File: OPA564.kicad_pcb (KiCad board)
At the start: 2 copper layers, 57.5 x 55 mm, 15 parts, among them IC1 OPA564AIDWD, J1 Conn_Coaxial, J2 Conn_Coaxial

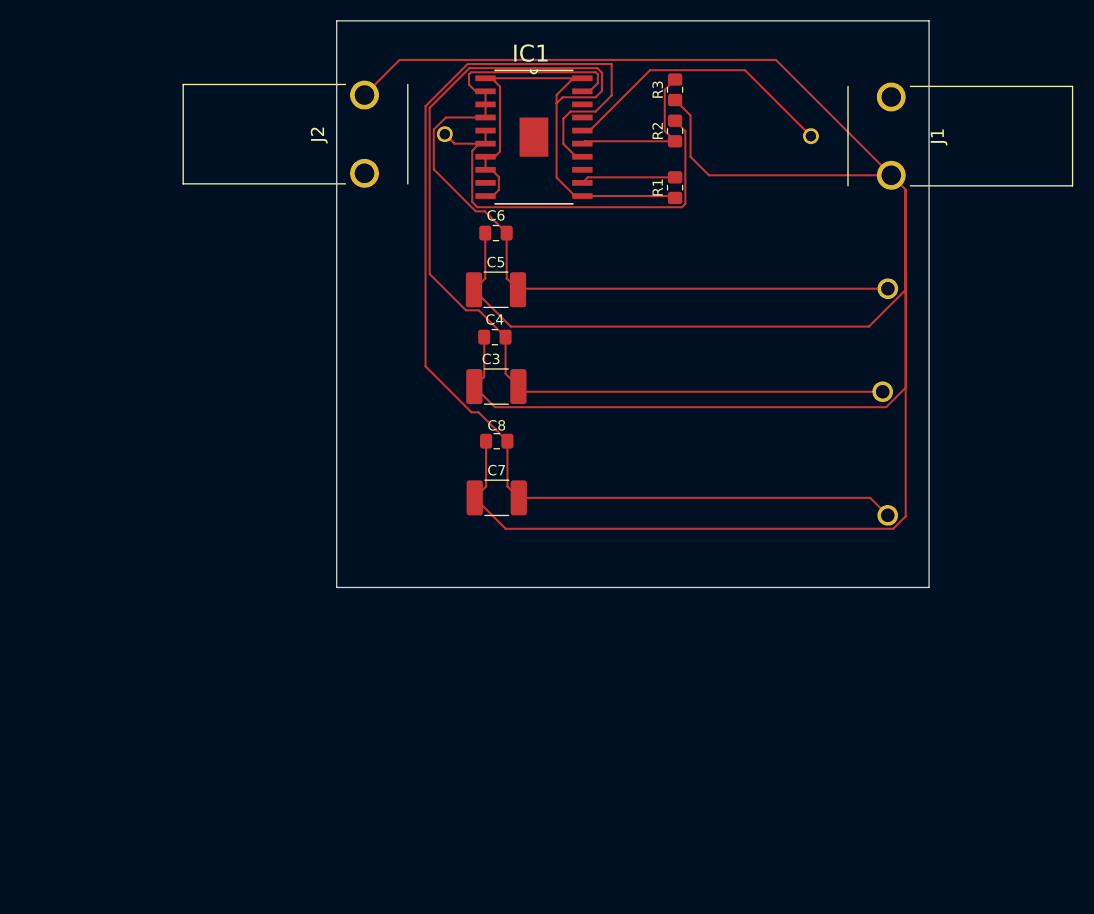
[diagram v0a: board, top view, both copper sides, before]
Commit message: zone areas
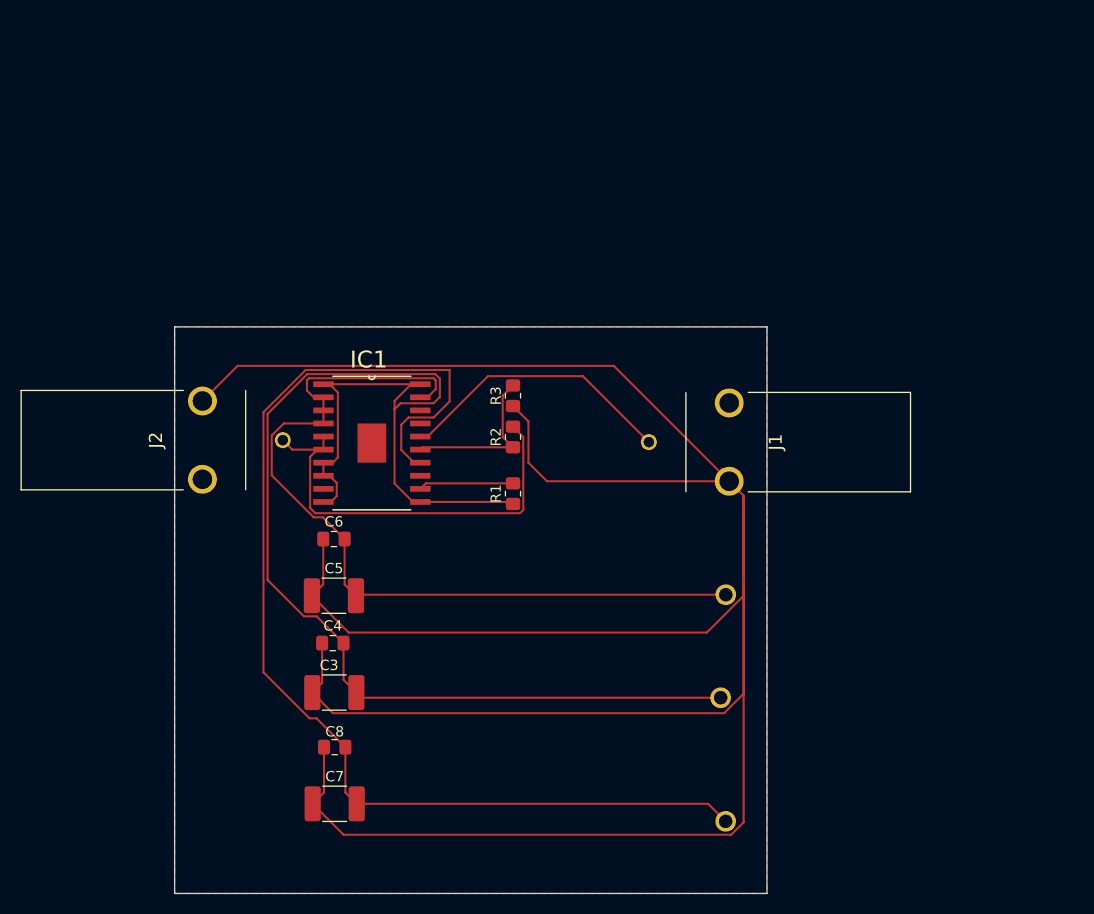
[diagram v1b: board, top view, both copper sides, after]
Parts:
- moved ? 33.6 mm to (169.8, 74.7)
- moved ? 33.6 mm to (169.8, 96.7)
- moved ? 33.6 mm to (169.3, 84.7)
- moved C3 33.6 mm to (131.8, 84.2)
- moved C4 33.6 mm to (131.6, 79.4)
- moved C7 33.6 mm to (131.8, 95.0)
- moved C8 33.6 mm to (131.8, 89.5)
- moved J1 33.6 mm to (162.3, 59.9)
- moved J2 33.6 mm to (126.8, 59.7)
- moved R1 33.6 mm to (149.1, 64.9)
- moved R2 33.6 mm to (149.1, 59.4)
- moved R3 33.6 mm to (149.1, 55.4)
- moved C5 33.6 mm to (131.7, 74.8)
- moved C6 33.6 mm to (131.7, 69.3)
- moved IC1 33.6 mm to (135.4, 60.0)
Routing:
- added copper zone on F.Cu, net GND
